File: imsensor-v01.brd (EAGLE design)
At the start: 53 x 46 mm, 13 parts, among them J1-A3 PJ-313-SPAD, J2-A2 PJ-313-SPAD, J3-A1 PJ-313-SPAD, J4-D3 PJ-313-SPAD, J5-D5 PJ-313-SPAD, J6-D6 PJ-313-SPAD, U1 ARDUINO_SHIELDNO_SILK

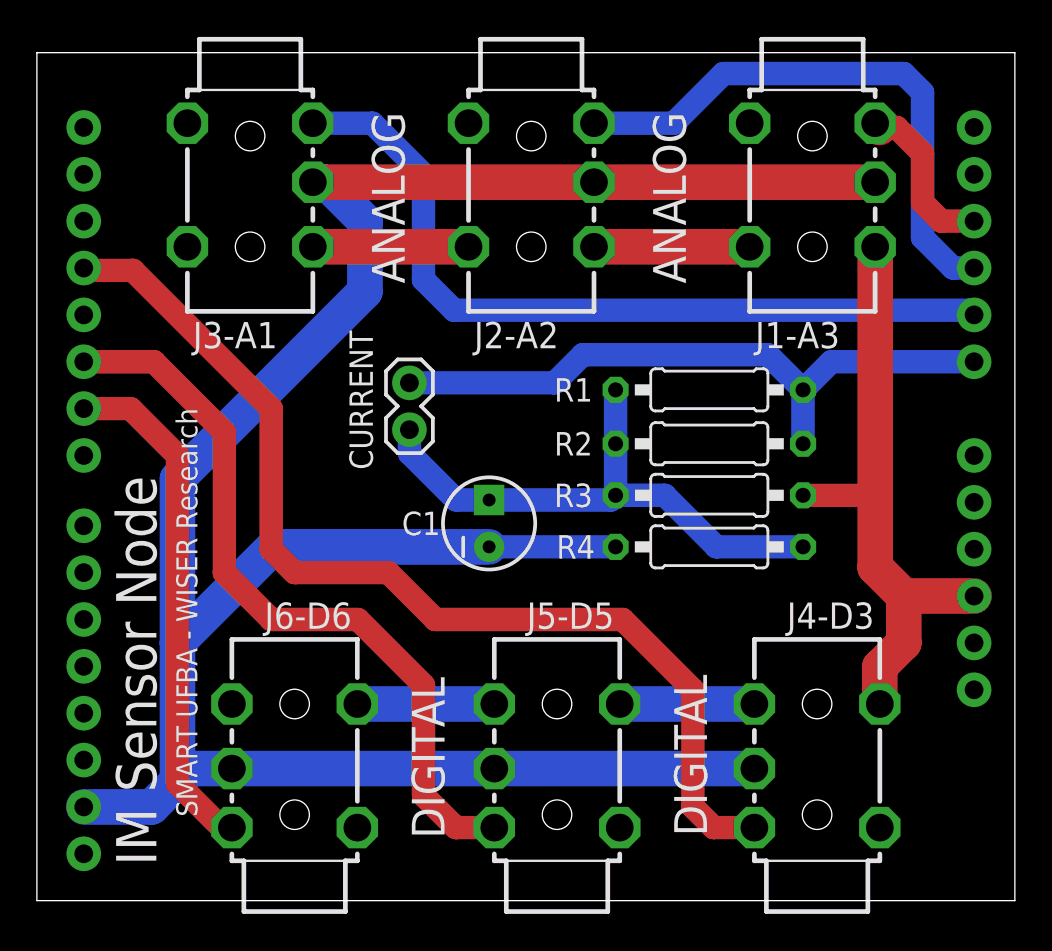
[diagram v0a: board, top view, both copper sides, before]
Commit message: IM Sensor Node v0.2
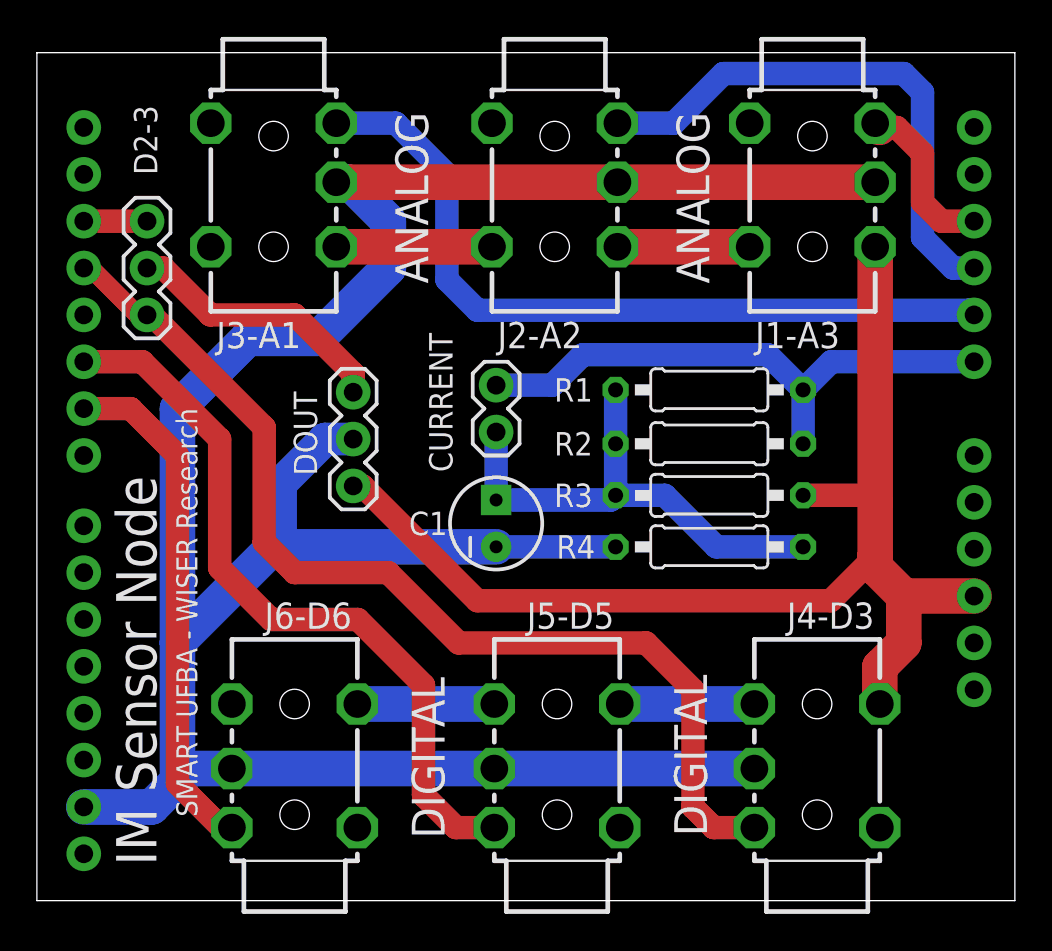
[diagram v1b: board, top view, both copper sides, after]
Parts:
- added D2-3, DOUT: (no value), SparkFun-Connectors:1X03
- moved CURRENT 4.70 mm to (24.9, 25.4)
- moved J2-A2 1.27 mm to (28.1, 43.9)
- moved J3-A1 1.27 mm to (12.8, 43.9)
- moved C1 0.38 mm to (24.9, 20.4)
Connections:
- new net N$13: D2-3.1, J4-D3.1.1, U1.D3
- new net N$14: D2-3.3, U1.D2
- net GND: now also DOUT.2
- net N$8: now also D2-3.2, DOUT.3; no longer J4-D3.1.1, U1.D3
- net VCC: now also DOUT.1
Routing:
- net N$13: track 0.00 -> 56.3 mm
- net N$8: track 57.1 -> 14.6 mm
- net VCC: track 33.8 -> 65.7 mm
- net GND: track 131.9 -> 141.8 mm
- net N$10: track 35.6 -> 30.9 mm
- net N$14: track 0.00 -> 3.43 mm
- net N$11: track 30.6 -> 27.3 mm
- net N$4: track 30.7 -> 29.4 mm
- net N$1: track 8.44 -> 7.17 mm
- net N$5: track 43.5 -> 42.2 mm
